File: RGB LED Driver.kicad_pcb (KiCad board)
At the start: 2 copper layers, 97.5 x 79 mm, 140 parts, among them J1 USB_C_Receptacle_USB2.0, J2 Conn_01x06_Pin, Q1 AO3400A, Q2 AO3400A, Q3 AO3400A, Q4 AO3400A, SW1 BOOT, U1 TPS61170DRVR, U10 LM358, U2 AP2112K-3.3TRG1, U3 LM358, U4 USBLC6-2SC6, U5 CP2104-F03-GM, U6 ESP32-WROOM-32, U7 CMXT3904, U8 LM358, U9 LM358

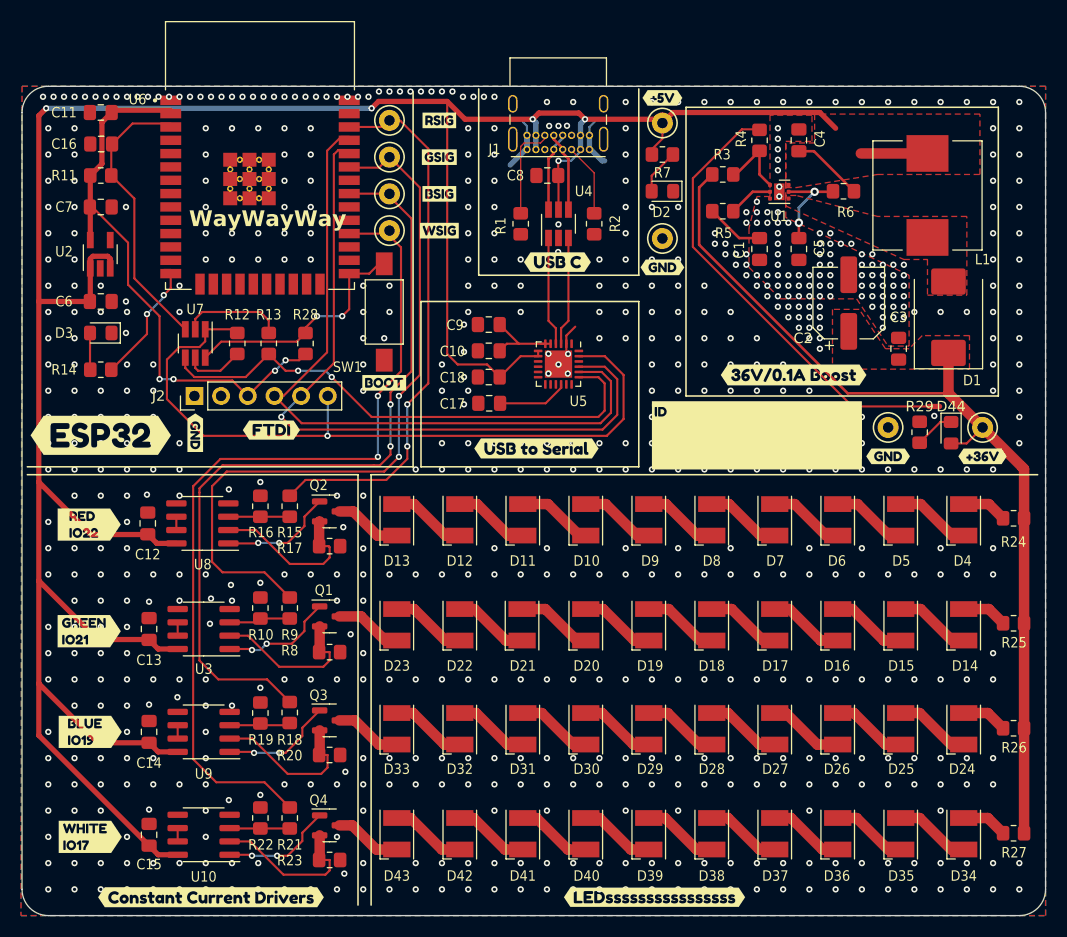
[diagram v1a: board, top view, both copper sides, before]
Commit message: updated pcb with BOM
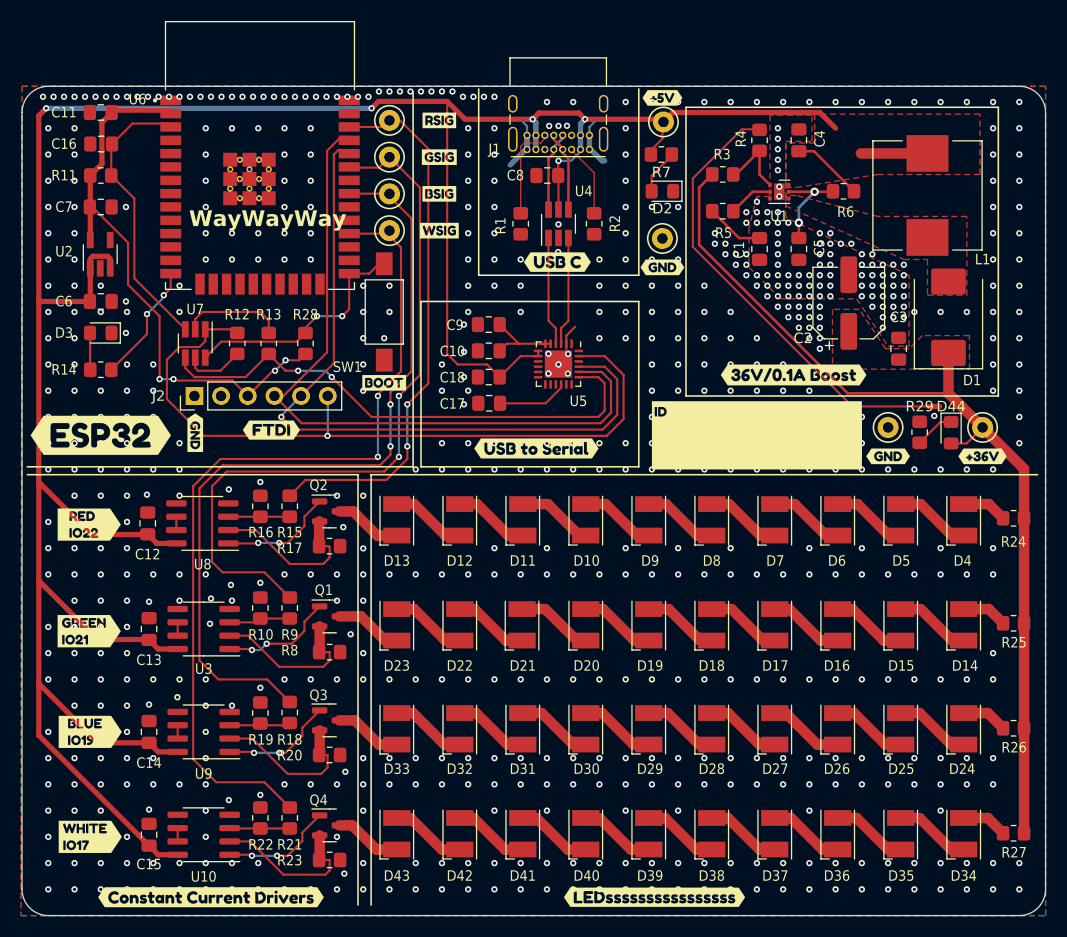
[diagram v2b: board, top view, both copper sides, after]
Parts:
- C17: value 1uF -> 4.7uF
- C2: value 10uF -> 10uF/63V
- C9: value 100nf -> 100nF
- D1: value SS35 -> SS36
- D3: value LED -> RED LED
- J1: value USB_C_Receptacle_USB2.0 -> USB4085
- NT1: value NetTie_2 -> Nettie
- R10, R16, R19, R22: value 5.1K -> 51K
- R14: value 1K -> 2K
- R17, R20, R23, R8: value 22R -> 100R
- R4: value 10.5K -> 10K/1%
- moved TP1 0.14 mm to (143.6, 56.9)
- moved R7 0.10 mm to (143.4, 60.0)
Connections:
- net /ESP32/LED_B renamed /BSig
- net /ESP32/LED_G renamed /GSig
- net /ESP32/LED_R renamed /RSig
- net /ESP32/LED_W renamed /WSig
- net Net-(J1-D+-PadA6) renamed /USB_C/USB_IN_P
- net Net-(J1-D--PadA7) renamed /USB_C/USB_IN_N
- net Net-(Q1-S) renamed /LED Driver G/Ifb
- net Net-(Q2-S) renamed /LED Driver R/Ifb
- net Net-(Q3-S) renamed /LED Driver B/Ifb
- net Net-(Q4-S) renamed /LED Driver W/Ifb
- net Net-(U10A-+) renamed /LED Driver W/VSet_2V0
- net Net-(U3A-+) renamed /LED Driver G/VSet_2V0
- net Net-(U8A-+) renamed /LED Driver R/VSet_2V0
- net Net-(U9A-+) renamed /LED Driver B/VSet_2V0
